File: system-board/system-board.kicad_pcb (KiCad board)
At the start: 4 copper layers, 50 x 16 mm, 67 parts, among them IC1 Flash_16Mb, IC2 LSM6DSLTR, IC3 NCP186AMX330TAG, IC4 MCP73834T-FCI_MF, J1 BATT, J11 503398-1892, J2 LEDs, J3 QWIIC, J4 SPKR, J5 105450-0101, J9 BTNs, Q1 DMP1012UFDF, Q2 SSM6K504NU.LF, Q3 SSM6K504NU.LF, Q4 DMP1012UFDF, Q5 PMZB290UNE2YL, Q6 PMZB290UNE2YL, Q7 PMZB290UNE2YL, Q8 PMZB290UNE2YL, SW1 RST, SW2 USR, U1 MDBT50Q-1MV2, U2 MAX98357AETE+T, U3 BQ29705DSER, Y1 32.768k

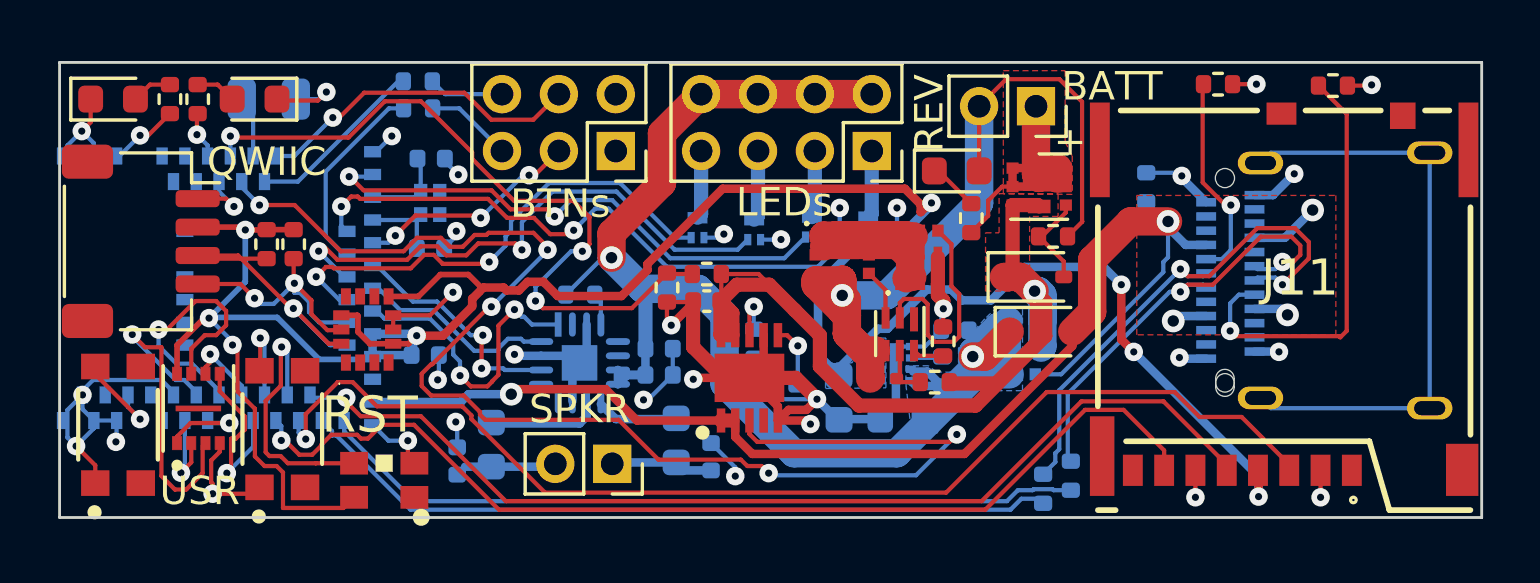
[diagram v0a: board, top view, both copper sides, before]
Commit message: Yet another PCB Revision
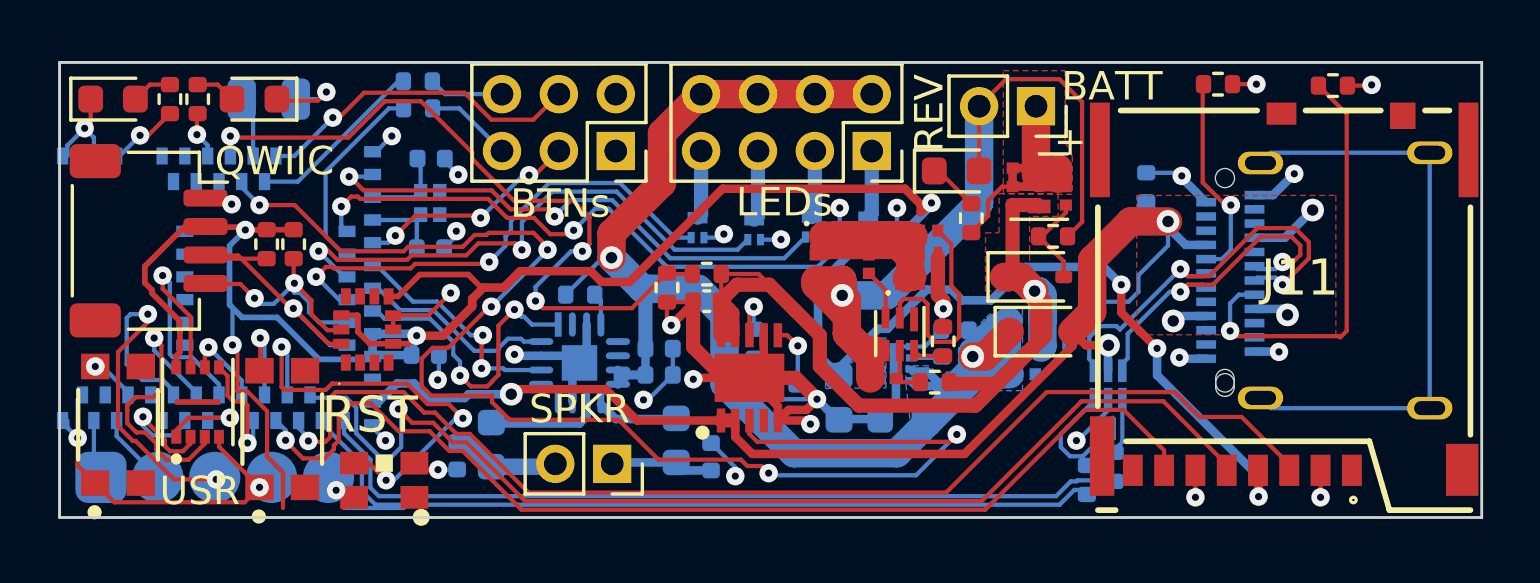
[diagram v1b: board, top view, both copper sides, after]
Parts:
- added IC5: HSP061-2M6, Imports:SON50P100X145X65-6N-D, B.Cu at (104.1, 103.9)
- added J6: DBG, Imports:Prog-Pads, B.Cu at (72.7, 107.2)
- moved R2 1.57 mm to (103.3, 107.2)
- moved R1 1.57 mm to (104.3, 106.8)
- moved J3 0.28 mm to (70.4, 98.8)
- moved IC1 0.23 mm to (72.1, 104.5)
- moved C5 0.18 mm to (81.2, 106.4), turned to 90 degrees
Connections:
- J5 pad A6: /CONN_USB_D+ -> /USB Connector/RAW_D+
- J5 pad A7: /CONN_USB_D- -> /USB Connector/RAW_D-
- J5 pad B6: /CONN_USB_D+ -> /USB Connector/RAW_D+
- J5 pad B7: /CONN_USB_D- -> /USB Connector/RAW_D-
- U1 pad 47: GND -> /SW0
- U1 pad 51: GND -> /SWDIO
- U1 pad 53: GND -> /SWCLK
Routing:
- net /USB Connector/RAW_D+: track 0.00 -> 15.1 mm, vias 0 -> 2
- net /CONN_USB_D-: track 16.1 -> 1.98 mm, vias 2 -> 0
- net /SW0: track 0.00 -> 13.1 mm, vias 0 -> 2
- net /USB Connector/RAW_D-: track 0.00 -> 12.2 mm, vias 0 -> 2
- net /CONN_USB_D+: track 18.8 -> 7.33 mm, vias 2 -> 0
- net /NEOPIX: track 8.97 -> 15.2 mm, vias 1 -> 3
- net /MCU_USB_D+: track 26.8 -> 31.0 mm
- net /Power Management/VBUS: track 50.0 -> 53.1 mm, vias 5 -> 6
- net /SWDIO: track 0.00 -> 2.60 mm
- net /SCK: track 36.2 -> 38.8 mm
- net /QSPI_D0: track 6.46 -> 4.15 mm
- net /MCU_USB_D-: track 27.1 -> 29.3 mm
- net /SWCLK: track 0.00 -> 1.75 mm
- net /QSPI_D1: track 3.09 -> 4.79 mm
- net /SWITCH: track 3.25 -> 1.62 mm
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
